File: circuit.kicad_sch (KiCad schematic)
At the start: 70 parts, among them J1 ???, J2 CTX 3V3 GND TX, J3 CRX 3V3 GND RX, J4 PICO GP4/GP5 CAN, J5 USB-C, Q1 PMV100EPAR, U1 SN65HVD230DR, U2 AMS1117

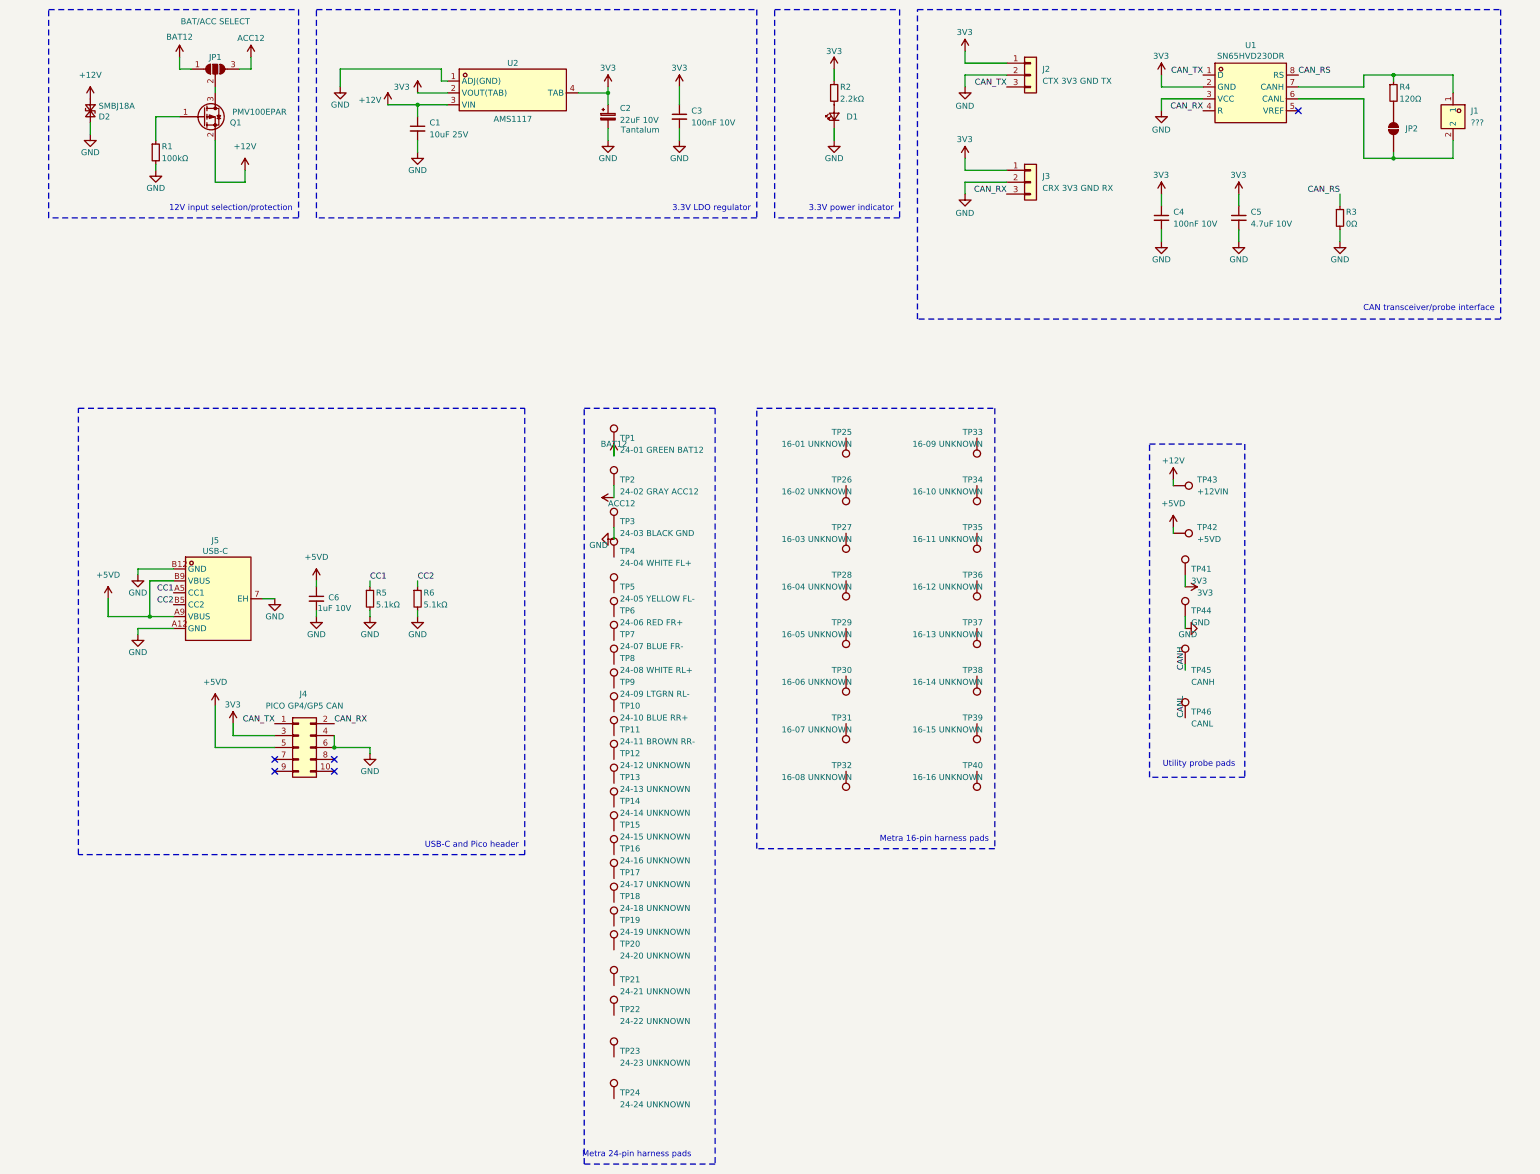
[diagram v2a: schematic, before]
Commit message: progress
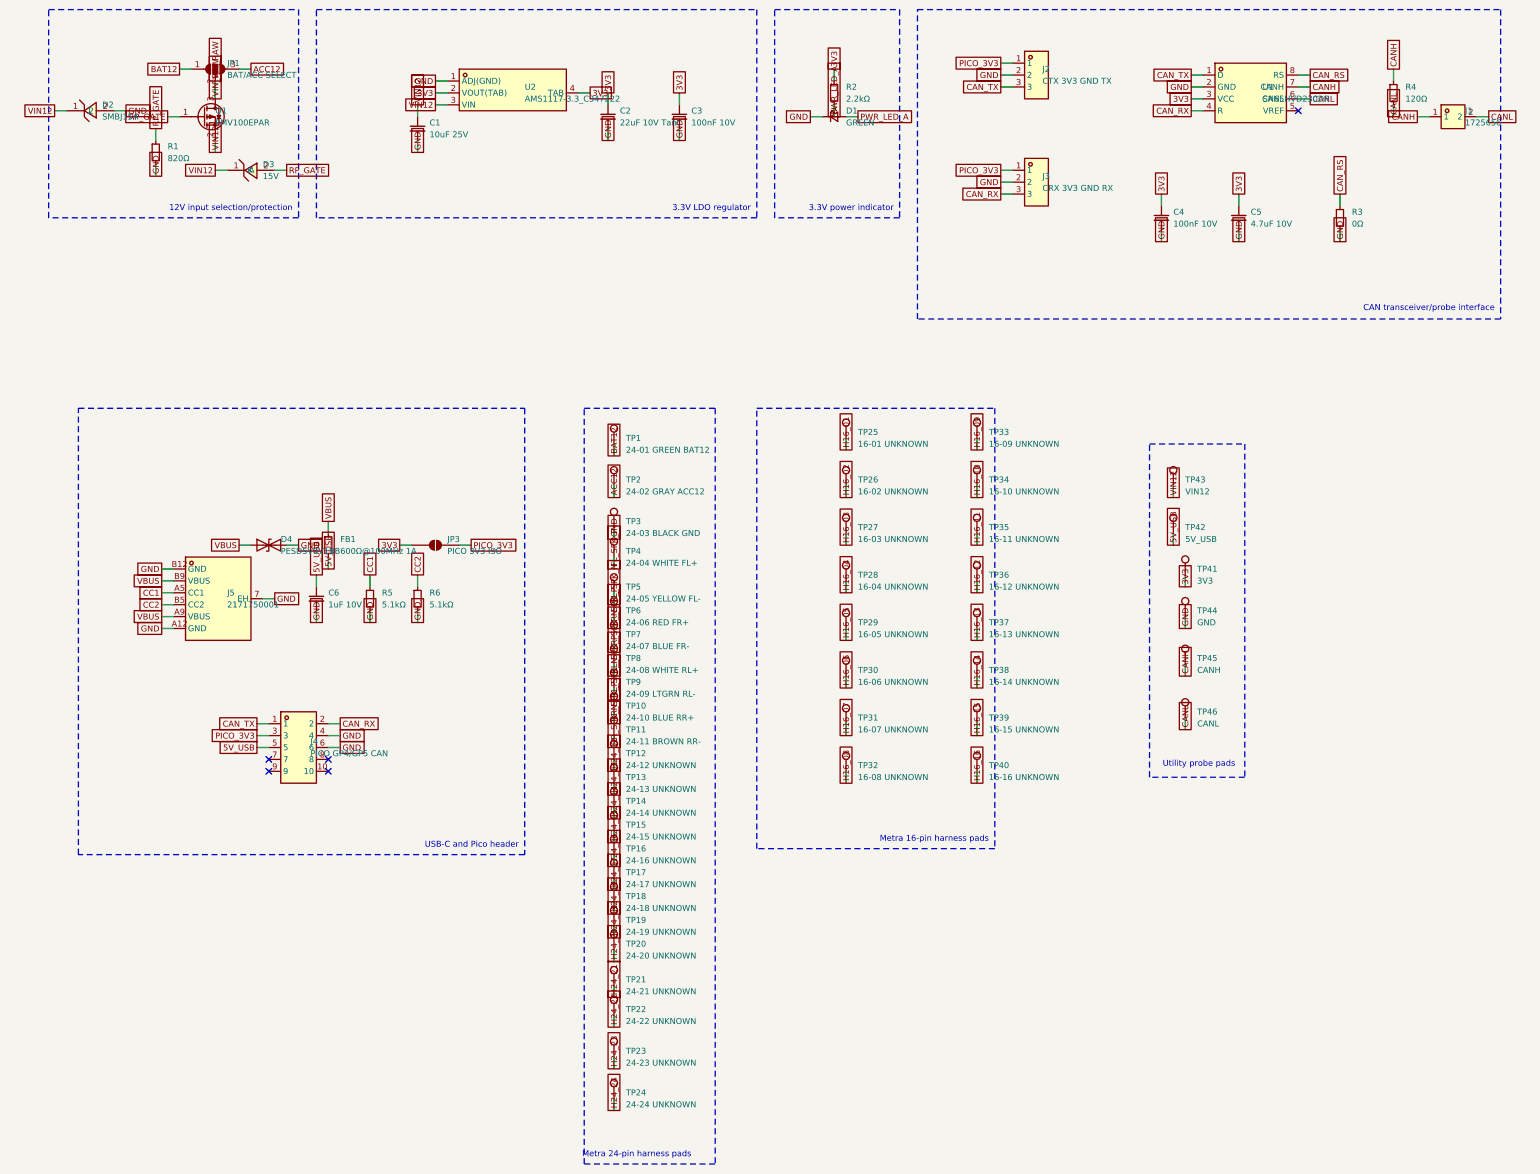
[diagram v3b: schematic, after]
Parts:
- removed C2: 22uF 10V, Capacitor_Tantalum_SMD:CP_EIA-3528-21_Kemet-B_HandSolder, symbol Device:C_Polarized_Small
- removed D1: Green LED, LED_SMD:LED_0603_1608Metric, symbol Device:LED_Small
- removed D2: SMBJ18A, Diode_SMD:D_SMB, symbol Device:D_TVS_Small
- removed J2: CTX 3V3 GND TX, Connector_PinHeader_2.54mm:PinHeader_1x03_P2.54mm_Vertical, symbol Connector_Generic:Conn_01x03
- removed J3: CRX 3V3 GND RX, Connector_PinHeader_2.54mm:PinHeader_1x03_P2.54mm_Vertical, symbol Connector_Generic:Conn_01x03
- removed J4: PICO GP4/GP5 CAN, Connector_PinHeader_2.54mm:PinHeader_2x05_P2.54mm_Vertical, symbol Connector_Generic:Conn_02x05_Odd_Even
- removed JP2: TERM OPEN, Jumper:SolderJumper-2_P1.3mm_Open_RoundedPad1.0x1.5mm, symbol Jumper:SolderJumper_2_Open
- added C2: 22uF 10V Tant, Capacitor_Tantalum_SMD:CP_EIA-3528-21_Kemet-B_HandSolder, symbol Device:C_Small
- added D1: GREEN, LED_SMD:LED_0603_1608Metric, symbol Library:LED_Small
- added D2: SMBJ15A, Library:SMB_L4.6-W3.6-LS5.3-RD, symbol Library:SMBJ15A_C83846
- added D3: 15V, Library:SOD-123_L2.7-W1.6-LS3.7-RD, symbol Library:MMSZ5245BT1G
- added D4: PESD5V0V1BB, Library:SOD-523_L1.2-W0.8-LS1.6-RD, symbol Device:D_TVS
- added FB1: 600Ω@100MHz 1A, Resistor_SMD:R_0603_1608Metric, symbol Library:R_Small
- added J2: CTX 3V3 GND TX, Library:CONN-TH_705430002, symbol Library:705430002
- added J3: CRX 3V3 GND RX, Library:CONN-TH_705430002, symbol Library:705430002
- added J4: PICO GP4/GP5 CAN, Library:HDR-TH_10P-P2.54-V-M-R2-C5-S2.54, symbol Library:10897101
- added JP3: PICO 3V3 ISO, Jumper:SolderJumper-2_P1.3mm_Open_RoundedPad1.0x1.5mm, symbol Jumper:SolderJumper_2_Open
- J1: value ??? -> 1725656
- J5: value USB-C -> 2171750001
- R1: value 100kΩ -> 820Ω
- TP42: value +5VD -> 5V_USB
- TP43: value +12VIN -> VIN12
- U2: value AMS1117 -> AMS1117-3.3_C347222
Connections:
- net 3V3: now also U1.3 (VCC), C2.1, JP3.1 (A); no longer U1.2 (GND)
- net CANH: now also J1.1, R4.1, U1.7 (CANH)
- net CANL: now also J1.2, R4.2, U1.6 (CANL)
- net CAN_RX: now also J3.3, J4.2
- net CAN_TX: now also J2.3, J4.1
- net GND: now also U1.2 (GND), C2.2, D1.1 (K), D2.2, D4.2 (A2), J2.2, J3.2, J4.4, J4.6; no longer U1.3 (VCC)
- net RL_SPK_N: now reaches TP9.1
- net H16_01: now reaches TP25.1
- net H24_15: now reaches TP15.1
- net H16_15: now reaches TP39.1
- net H24_18: now reaches TP18.1
- net H24_16: now reaches TP16.1
- net RR_SPK_N: now reaches TP11.1
- net H24_13: now reaches TP13.1
- net H16_12: now reaches TP36.1
- net H24_19: now reaches TP19.1
- net PWR_LED_A: now reaches R2.2
- net PWR_LED_A: now also D1.2 (A)
- net H16_02: now reaches TP26.1
- net H24_23: now reaches TP23.1
- net H16_09: now reaches TP33.1
- net FL_SPK_N: now reaches TP5.1
- net H24_21: now reaches TP21.1
- net H24_17: now reaches TP17.1
- net H24_24: now reaches TP24.1
- net H16_04: now reaches TP28.1
- net FR_SPK_N: now reaches TP7.1
- net H16_07: now reaches TP31.1
- net H24_14: now reaches TP14.1
- net VIN_RAW: now reaches JP1.2 (C), Q1.3 (D)
- net FR_SPK_P: now reaches TP6.1
- net H24_20: now reaches TP20.1
- net H16_06: now reaches TP30.1
- net H24_12: now reaches TP12.1
- net FL_SPK_P: now reaches TP4.1
- net H16_10: now reaches TP34.1
- net H16_11: now reaches TP35.1
- net RL_SPK_P: now reaches TP8.1
- net H16_05: now reaches TP29.1
- net H24_22: now reaches TP22.1
- net RP_GATE: now reaches Q1.1 (G), R1.1
- net RP_GATE: now also D3.2 (A)
- net RR_SPK_P: now reaches TP10.1
- net H16_08: now reaches TP32.1
- net H16_16: now reaches TP40.1
- net H16_14: now reaches TP38.1
- net H16_13: now reaches TP37.1
- net H16_03: now reaches TP27.1
- net +12V renamed VIN12
- net VIN12: now also D2.1, D3.1 (K)
- net +5VD renamed 5V_USB
- net 5V_USB: now also FB1.2, J4.5; no longer J5.A9 (VBUS), J5.B9 (VBUS)
- new net PICO_3V3: J2.1, J3.1, J4.3, JP3.2 (B)
- new net VBUS: D4.1 (A1), FB1.1, J5.A9 (VBUS), J5.B9 (VBUS)
